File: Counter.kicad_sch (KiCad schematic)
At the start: 1 part, among them U1 74LS192

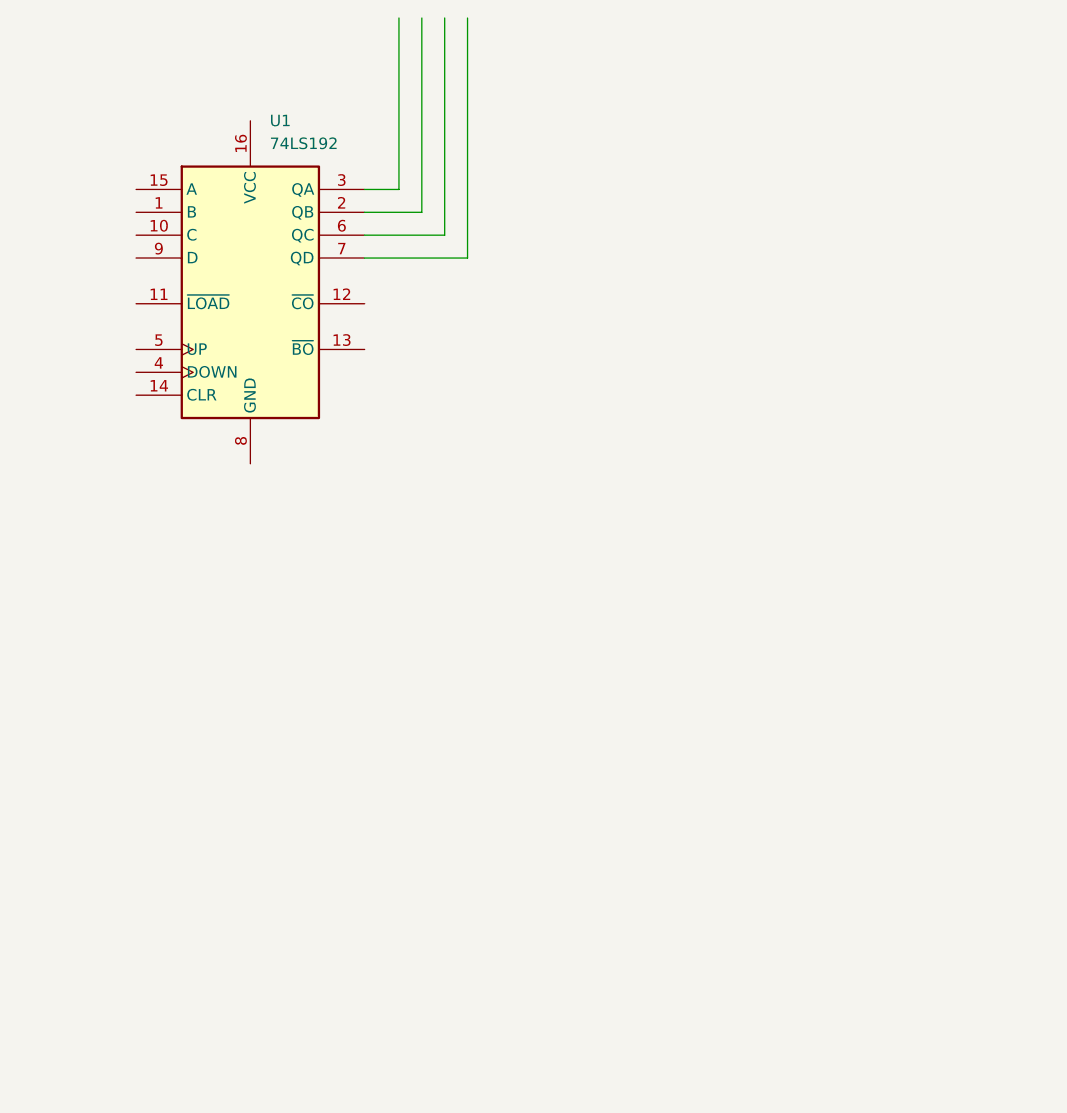
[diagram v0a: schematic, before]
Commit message: uodate
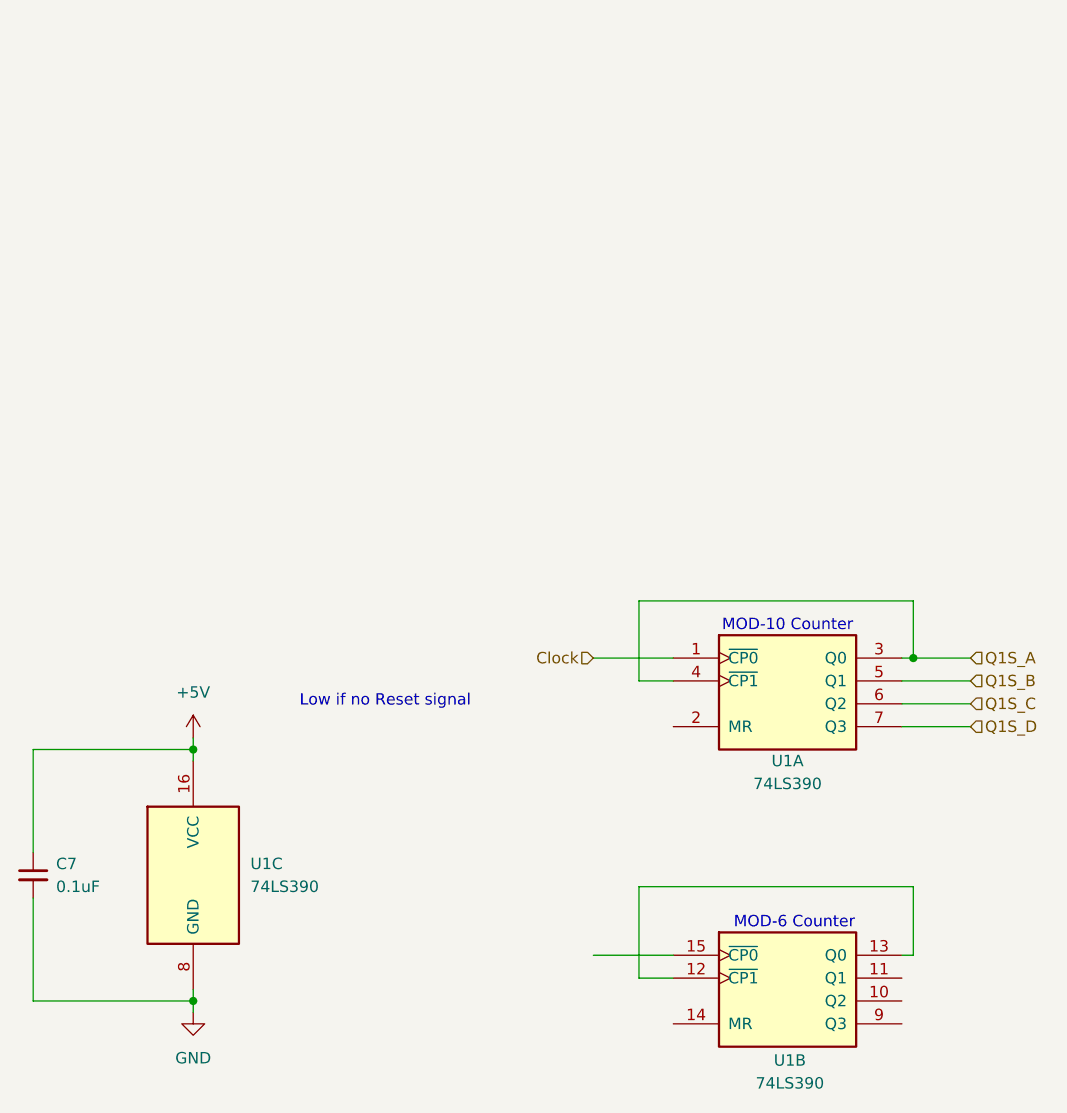
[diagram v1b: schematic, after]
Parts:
- removed U1: 74LS192, symbol 74xx:74LS192
- added C7: 0.1uF, symbol Device:C_Small
- added U1: 74LS390, symbol 74xx:74LS390
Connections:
- new net: U1.12 (~{CP1}), U1.13 (Q0)
- new net +5V: C7.1, U1.16 (VCC)
- new net Clock: U1.1 (~{CP0})
- new net GND: C7.2, U1.8 (GND)
- new net Q1S_A: U1.3 (Q0), U1.4 (~{CP1})
- new net Q1S_B: U1.5 (Q1)
- new net Q1S_C: U1.6 (Q2)
- new net Q1S_D: U1.7 (Q3)
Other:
- note added: "Low if no Reset signal"
- note added: "MOD-10 Counter"
- note added: "MOD-6 Counter"
